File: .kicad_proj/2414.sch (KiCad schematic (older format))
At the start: 1 part, among them U1 ATmega328-PU

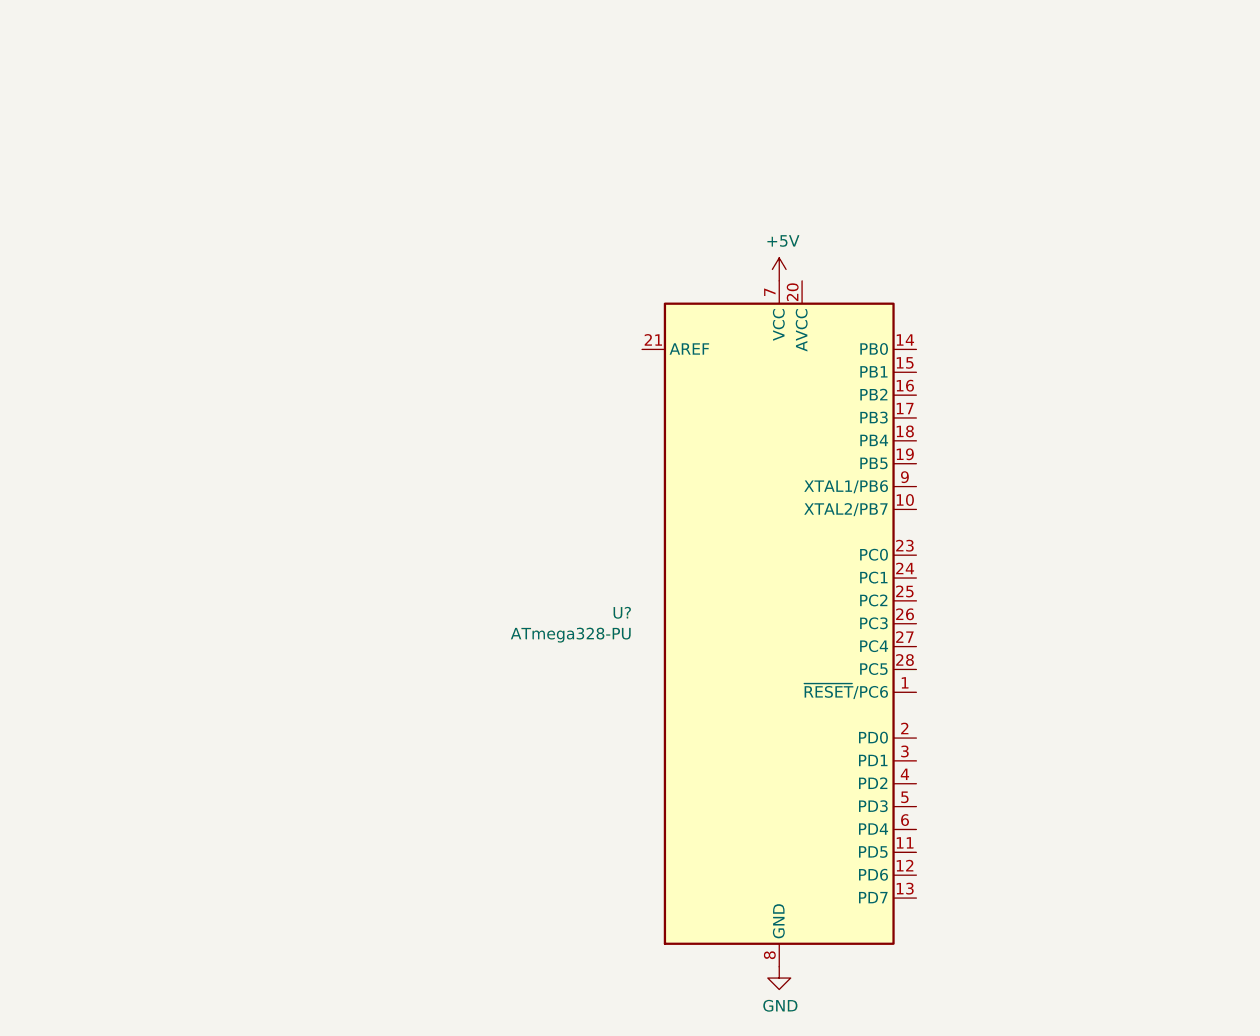
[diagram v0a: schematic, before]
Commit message: Finish schematics 14-16
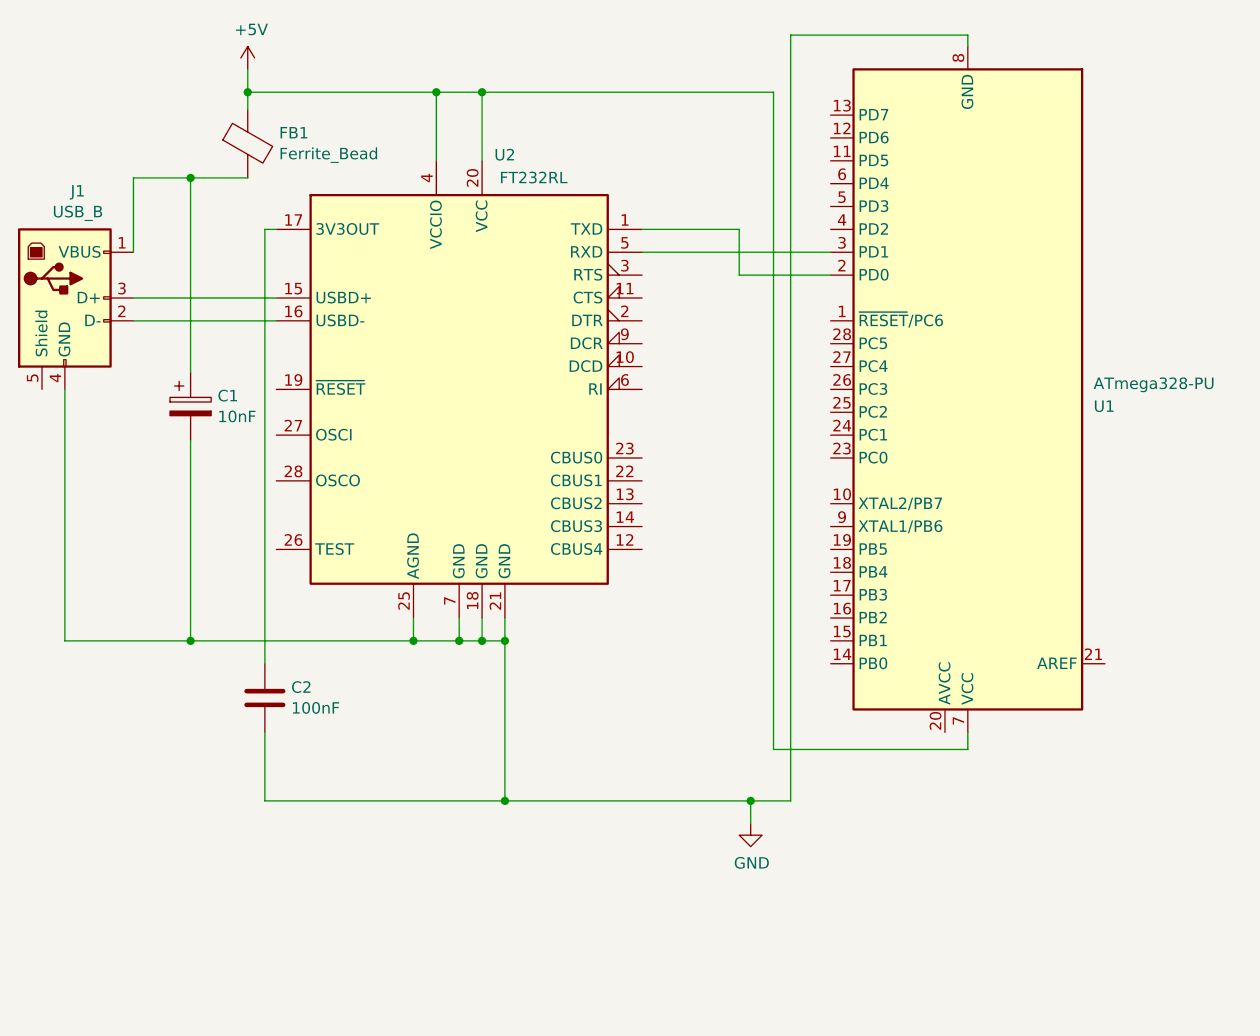
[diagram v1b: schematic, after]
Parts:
- added C1: 10nF, symbol Device:CP
- added C2: 100nF, symbol Device:C
- added FB1: Ferrite_Bead, symbol Device:Ferrite_Bead
- added J1: USB_B, symbol Connector:USB_B
- added U2: FT232RL, Package_SO:SSOP-28_5.3x10.2mm_P0.65mm, symbol Interface_USB:FT232RL
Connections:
- net +5V: now also FB1.1, U2.20 (VCC), U2.4 (VCCIO)
- net GND: now also C1.2, C2.2, J1.4 (GND), U2.18 (GND), U2.21 (GND), U2.25 (AGND), U2.7 (GND)
- net at U1.2 (PD0): now also U2.1 (TXD)
- net at U1.3 (PD1): now also U2.5 (RXD)
- new net: J1.3 (D+), U2.15 (USBD+)
- new net: J1.2 (D-), U2.16 (USBD-)
- new net: C2.1, U2.17 (3V3OUT)
- new net: C1.1, FB1.2, J1.1 (VBUS)
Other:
- moved on the sheet: U1
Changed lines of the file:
@@
 L MCU_Microchip_ATmega:ATmega328-PU U?
 U 1 1 60A417FE
-P 4950 3500
+P 5775 2475
 AR Path="/60A417FE" Ref="U?"  Part="1"
 AR Path="/607B2C9D/60A417FE" Ref="U1"  Part="1"
 AR Path="/60A3FFA8/60A417FE" Ref="U?"  Part="1"
 AR Path="/60A4150D/60A417FE" Ref="U?"  Part="1"
-AR Path="/60A41615/60A417FE" Ref="U?"  Part="1"
-F 0 "U?" H 4306 3546 50  0000 R CNN
-F 1 "ATmega328-PU" H 4306 3455 50  0000 R CNN
-F 2 "Package_DIP:DIP-28_W7.62mm" H 4950 3500 50  0001 C CIN
-F 3 "http://ww1.microchip.com/downloads/en/DeviceDoc/ATmega328_P%20AVR%20MCU%20with%20picoPower%20Technology%20Data%20Sheet%2040001984A.pdf" H 4950 3500 50  0001 C CNN
-	1    4950 3500
-	1    0    0    -1
+AR Path="/60A41615/60A417FE" Ref="U1"  Part="1"
+F 0 "U1" H 5225 2550 50  0000 R CNN
+F 1 "ATmega328-PU" H 5225 2450 50  0000 R CNN
+F 2 "Package_DIP:DIP-28_W7.62mm" H 5775 2475 50  0001 C CIN
+F 3 "http://ww1.microchip.com/downloads/en/DeviceDoc/ATmega328_P%20AVR%20MCU%20with%20picoPower%20Technology%20Data%20Sheet%2040001984A.pdf" H 5775 2475 50  0001 C CNN
+	1    5775 2475
+	-1   0    0    1
 $EndComp
 $Comp
 L power:GND #PWR?
 U 1 1 60A417FA
-P 4950 5000
+P 4825 4375
 AR Path="/60A417FA" Ref="#PWR?"  Part="1"
 AR Path="/607B2C9D/60A417FA" Ref="#PWR?"  Part="1"
@@
 AR Path="/60A4150D/60A417FA" Ref="#PWR?"  Part="1"
 AR Path="/60A41615/60A417FA" Ref="#PWR?"  Part="1"
-F 0 "#PWR?" H 4950 4750 50  0001 C CNN
-F 1 "GND" H 4955 4827 50  0000 C CNN
-F 2 "" H 4950 5000 50  0001 C CNN
-F 3 "" H 4950 5000 50  0001 C CNN
-	1    4950 5000
+F 0 "#PWR?" H 4825 4125 50  0001 C CNN
+F 1 "GND" H 4830 4202 50  0000 C CNN
+F 2 "" H 4825 4375 50  0001 C CNN
+F 3 "" H 4825 4375 50  0001 C CNN
+	1    4825 4375
+	1    0    0    -1
+$EndComp
+$Comp
+L Interface_USB:FT232RL U2
+U 1 1 60B487A5
+P 3550 2475
+F 0 "U2" H 3750 3500 50  0000 C CNN
+F 1 "FT232RL" H 3875 3400 50  0000 C CNN
+F 2 "Package_SO:SSOP-28_5.3x10.2mm_P0.65mm" H 4650 1575 50  0001 C CNN
+F 3 "https://www.ftdichip.com/Support/Documents/DataSheets/ICs/DS_FT232R.pdf" H 3550 2475 50  0001 C CNN
+	1    3550 2475
 	1    0    0    -1
 $EndComp
@@
 L power:+5V #PWR?
 U 1 1 60A417FC
-P 4950 2000
+P 2625 1075
 AR Path="/60A417FC" Ref="#PWR?"  Part="1"
 AR Path="/607B2C9D/60A417FC" Ref="#PWR?"  Part="1"
@@
 AR Path="/60A4150D/60A417FC" Ref="#PWR?"  Part="1"
 AR Path="/60A41615/60A417FC" Ref="#PWR?"  Part="1"
-F 0 "#PWR?" H 4950 1850 50  0001 C CNN
-F 1 "+5V" H 4965 2173 50  0000 C CNN
-F 2 "" H 4950 2000 50  0001 C CNN
-F 3 "" H 4950 2000 50  0001 C CNN
-	1    4950 2000
+F 0 "#PWR?" H 2625 925 50  0001 C CNN
+F 1 "+5V" H 2640 1248 50  0000 C CNN
+F 2 "" H 2625 1075 50  0001 C CNN
+F 3 "" H 2625 1075 50  0001 C CNN
+	1    2625 1075
 	1    0    0    -1
 $EndComp
+Wire Wire Line
+	4350 1775 4775 1775
+Wire Wire Line
+	4775 1975 5175 1975
+Wire Wire Line
+	4775 1775 4775 1975
+Wire Wire Line
+	4350 1875 5175 1875
+Wire Wire Line
+	4825 4375 4825 4275
+Wire Wire Line
+	5775 925  5775 975
+Wire Wire Line
+	4825 4275 3750 4275
+Wire Wire Line
+	3750 4275 3750 3575
+Connection ~ 4825 4275
+Wire Wire Line
+	3650 3475 3650 3575
+Wire Wire Line
+	3650 3575 3750 3575
+Connection ~ 3750 3575
+Wire Wire Line
+	3750 3575 3750 3475
+Wire Wire Line
+	3650 3575 3550 3575
+Wire Wire Line
+	3350 3575 3350 3475
+Connection ~ 3650 3575
+Wire Wire Line
+	3550 3475 3550 3575
+Connection ~ 3550 3575
+Wire Wire Line
+	3550 3575 3350 3575
+Wire Wire Line
+	3650 1475 3650 1175
+Wire Wire Line
+	3650 1175 3450 1175
+Wire Wire Line
+	3450 1475 3450 1175
+Connection ~ 3450 1175
+Wire Wire Line
+	3450 1175 2625 1175
+$Comp
+L Connector:USB_B J1
+U 1 1 60B801EF
+P 1825 2075
+F 0 "J1" H 1882 2542 50  0000 C CNN
+F 1 "USB_B" H 1882 2451 50  0000 C CNN
+F 2 "" H 1975 2025 50  0001 C CNN
+F 3 " ~" H 1975 2025 50  0001 C CNN
+	1    1825 2075
+	1    0    0    -1
+$EndComp
+$Comp
+L Device:Ferrite_Bead FB1
+U 1 1 60B831C7
+P 2625 1400
+F 0 "FB1" H 2762 1446 50  0000 L CNN
+F 1 "Ferrite_Bead" H 2762 1355 50  0000 L CNN
+F 2 "" V 2555 1400 50  0001 C CNN
+F 3 "~" H 2625 1400 50  0001 C CNN
+	1    2625 1400
+	1    0    0    -1
+$EndComp
+Wire Wire Line
+	2625 1075 2625 1175
+Connection ~ 2625 1175
+Wire Wire Line
+	2625 1175 2625 1250
+Wire Wire Line
+	2625 1550 2375 1550
+Wire Wire Line
+	2125 1550 2125 1875
+Wire Wire Line
+	3350 3575 2375 3575
+Wire Wire Line
+	1825 3575 1825 2475
+Connection ~ 3350 3575
+$Comp
+L Device:C C2
+U 1 1 60B856CC
+P 2700 3825
+F 0 "C2" H 2815 3871 50  0000 L CNN
+F 1 "100nF" H 2815 3780 50  0000 L CNN
+F 2 "" H 2738 3675 50  0001 C CNN
+F 3 "~" H 2700 3825 50  0001 C CNN
+	1    2700 3825
+	1    0    0    -1
+$EndComp
+Wire Wire Line
+	2375 2400 2375 1550
+Connection ~ 2375 1550
+Wire Wire Line
+	2375 1550 2125 1550
+Wire Wire Line
+	2375 2700 2375 3575
+Connection ~ 2375 3575
+Wire Wire Line
+	2375 3575 1825 3575
+$Comp
+L Device:CP C1
+U 1 1 60B8A756
+P 2375 2550
+F 0 "C1" H 2493 2596 50  0000 L CNN
+F 1 "10nF" H 2493 2505 50  0000 L CNN
+F 2 "" H 2413 2400 50  0001 C CNN
+F 3 "~" H 2375 2550 50  0001 C CNN
+	1    2375 2550
+	1    0    0    -1
+$EndComp
+Wire Wire Line
+	2750 2075 2125 2075
+Wire Wire Line
+	2125 2175 2750 2175
+Wire Wire Line
+	2750 1775 2700 1775
+Wire Wire Line
+	2700 1775 2700 3675
+Wire Wire Line
+	2700 3975 2700 4275
+Wire Wire Line
+	2700 4275 3750 4275
+Connection ~ 3750 4275
+Wire Wire Line
+	3650 1175 4925 1175
+Connection ~ 3650 1175
+Wire Wire Line
+	4825 4275 5000 4275
+Wire Wire Line
+	4925 1175 4925 4050
+Wire Wire Line
+	4925 4050 5775 4050
+Wire Wire Line
+	5775 4050 5775 3975
+Wire Wire Line
+	5000 4275 5000 925
+Wire Wire Line
+	5000 925  5775 925
 $EndSCHEMATC
